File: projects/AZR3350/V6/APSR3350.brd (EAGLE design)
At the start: 80.5 x 100 mm, 214 parts, among them IC1 A4403, IC10 A4988, IC2 LDO-TS1117CW-3V3, IC3 ATSAM4S8C, IC4 74AHC08, IC7 A4988, IC8 A4988, IC9 A4988, J1 ZX62-AB-5PA, J2 MOLEX-SD-47571-001, J3 MSTBV4, Q1 NX138BKS, Q2 AON7524, Q3 AON7524, Q4 BC817-16SMD, X1 12MHz

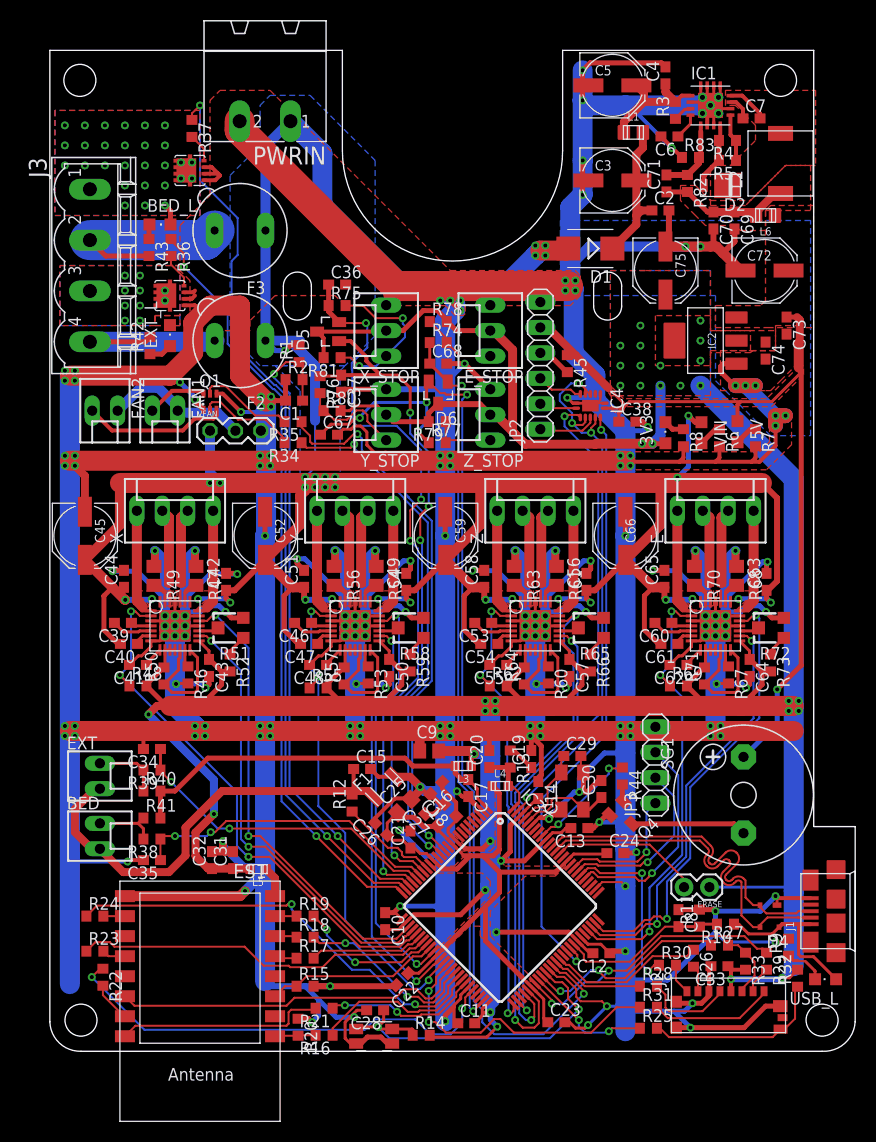
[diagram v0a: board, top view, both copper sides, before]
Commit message: Done**
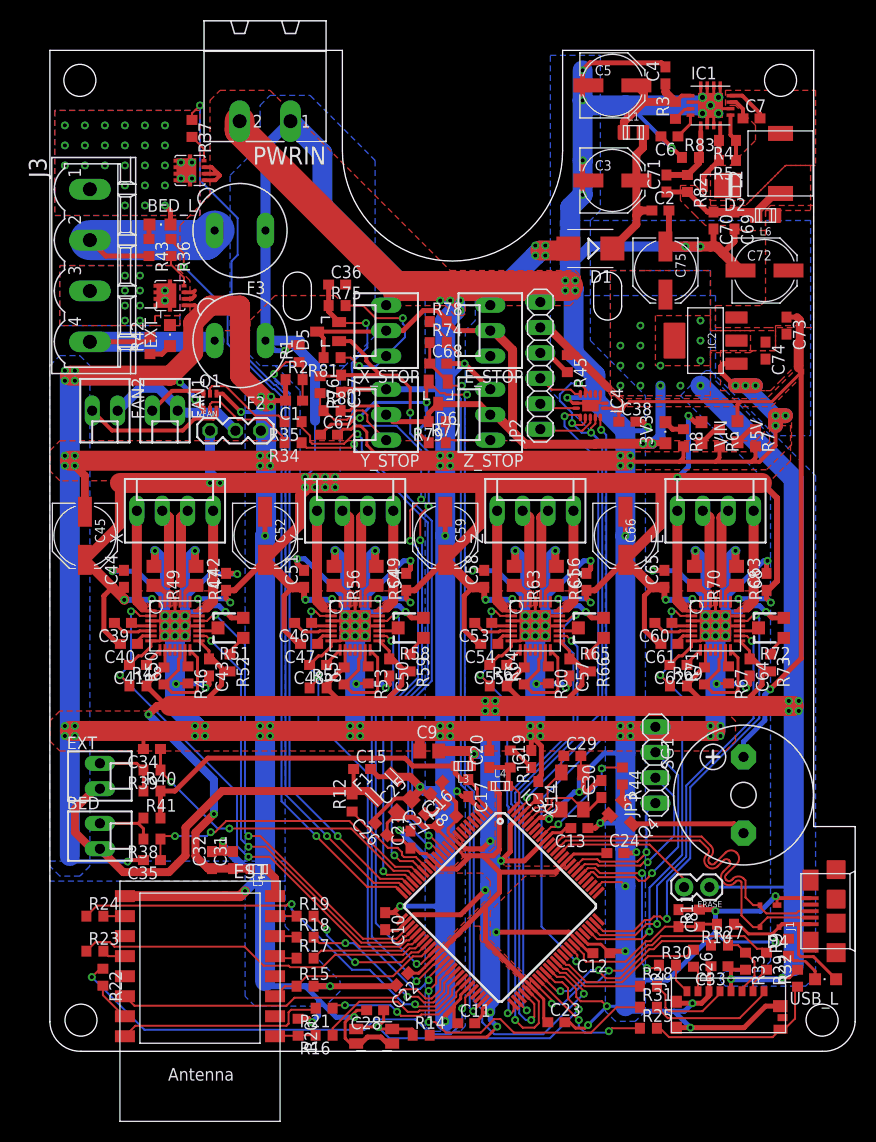
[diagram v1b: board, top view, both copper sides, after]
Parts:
- moved C43 0.05 mm to (15.9, 38.4)
- moved C50 0.05 mm to (33.9, 38.4)
- moved C57 0.05 mm to (51.9, 38.4)
- moved C64 0.05 mm to (69.9, 38.4)
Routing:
- net GND: track 1330.2 -> 1303.4 mm
- net +3V3: track 436.8 -> 438.0 mm
